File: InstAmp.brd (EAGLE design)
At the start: 77.5 x 18 mm, 37 parts, among them IC1 AD8221ARZ, IC2 TLC2254ID

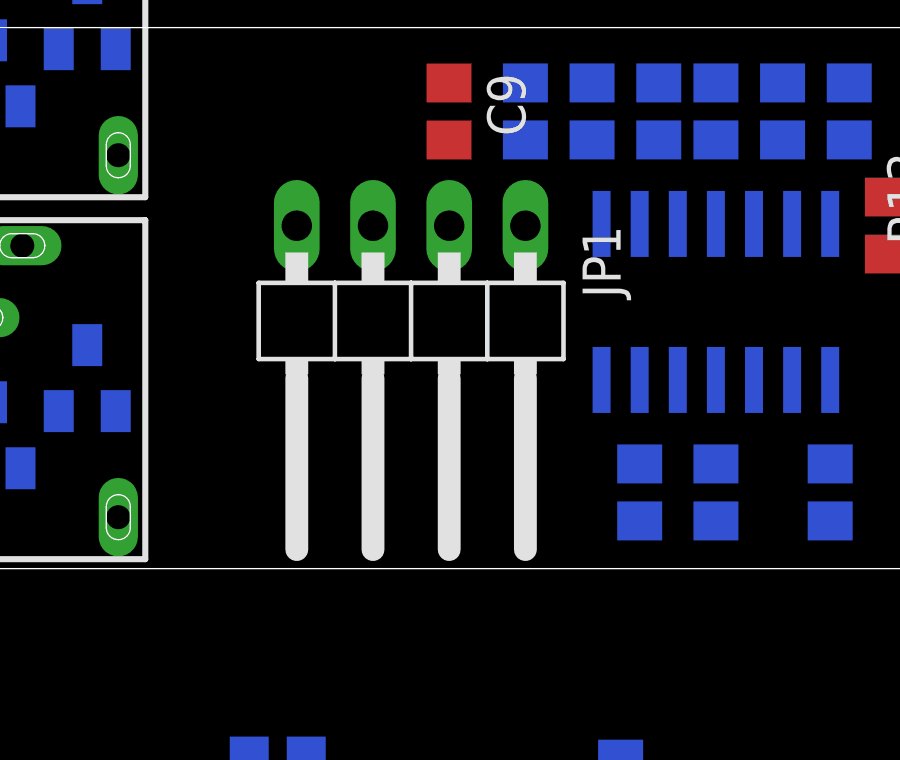
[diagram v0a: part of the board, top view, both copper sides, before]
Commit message: Amp routing
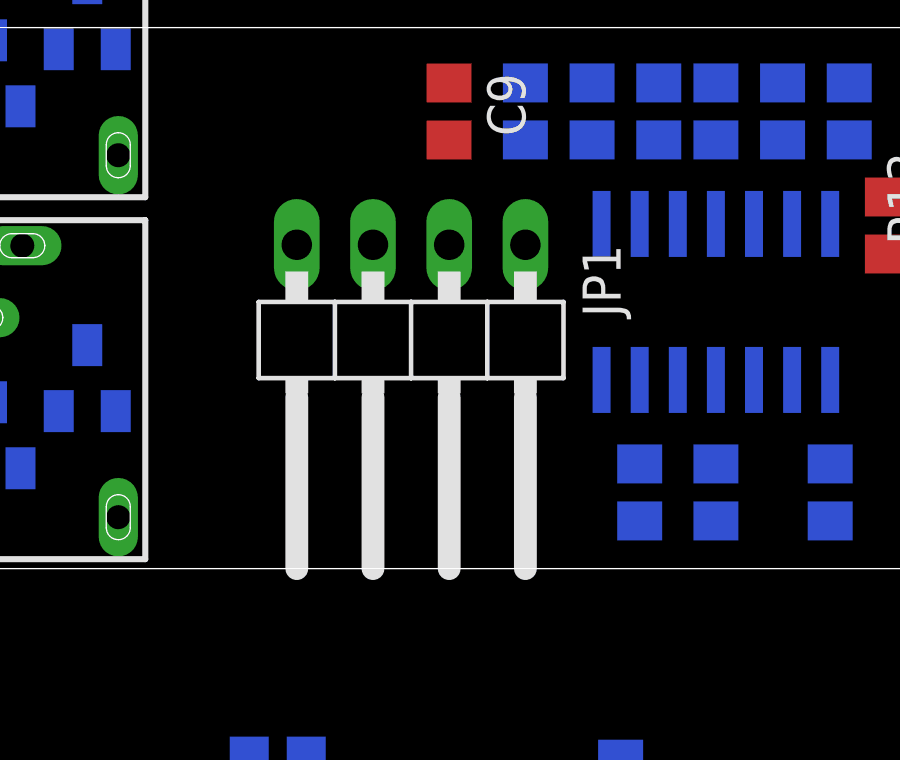
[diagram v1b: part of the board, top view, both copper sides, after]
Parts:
- moved JP1 0.63 mm to (22.9, 6.99)
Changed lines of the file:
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@@
 <element name="R16" library="rcl" package="R0805" value="910k" x="38.735" y="11.43" rot="R270"/>
 <element name="R17" library="rcl" package="R0805" value="100k" x="37.465" y="15.24" rot="MR270"/>
-<element name="JP1" library="pinhead" package="1X04/90" value="OUT" x="22.86" y="7.62" rot="R180"/>
+<element name="JP1" library="pinhead" package="1X04/90" value="OUT" x="22.86" y="6.985" rot="R180"/>
 <element name="IC2" library="linear" package="SO14" value="TLC2254ID" x="33.02" y="8.89" rot="MR180"/>
 </elements>
@@
 <wire x1="31.115" y1="16.19" x2="33.02" y2="16.19" width="0" layer="19" extent="16-16"/>
 <wire x1="28.8925" y1="16.19" x2="31.115" y2="16.19" width="0" layer="19" extent="16-16"/>
-<wire x1="24.13" y1="11.43" x2="28.8925" y2="16.19" width="0" layer="19" extent="16-16"/>
-<wire x1="30.48" y1="1.59" x2="24.13" y2="11.43" width="0" layer="19" extent="16-16"/>
+<wire x1="24.13" y1="10.795" x2="28.8925" y2="16.19" width="0" layer="19" extent="16-16"/>
+<wire x1="30.48" y1="1.59" x2="24.13" y2="10.795" width="0" layer="19" extent="16-16"/>
 <wire x1="33.02" y1="1.59" x2="30.48" y2="1.59" width="0" layer="19" extent="16-16"/>
 <wire x1="36.83" y1="1.59" x2="33.02" y2="1.59" width="0" layer="19" extent="16-16"/>
@@
 <wire x1="29.845" y1="-10.48" x2="29.845" y2="-8.2525" width="0" layer="19" extent="16-16"/>
 <wire x1="27.365" y1="-8.89" x2="29.845" y2="-8.2525" width="0" layer="19" extent="16-16"/>
-<wire x1="4.13" y1="5.715" x2="24.13" y2="11.43" width="0" layer="19" extent="16-16"/>
+<wire x1="4.13" y1="5.715" x2="24.13" y2="10.795" width="0" layer="19" extent="16-16"/>
 <wire x1="2.1" y1="5.715" x2="4.13" y2="5.715" width="0" layer="19" extent="16-16"/>
 <wire x1="4.13" y1="17.78" x2="4.13" y2="5.715" width="0" layer="19" extent="16-16"/>
@@
 <wire x1="29.845" y1="-6.3525" x2="33.02" y2="3.49" width="0" layer="19" extent="16-16"/>
 <wire x1="27.365" y1="-7.62" x2="29.845" y2="-6.3525" width="0" layer="19" extent="16-16"/>
-<wire x1="19.05" y1="11.43" x2="33.02" y2="6.29" width="0" layer="19" extent="16-16"/>
-<wire x1="13.015" y1="17.315" x2="19.05" y2="11.43" width="0" layer="19" extent="16-16"/>
+<wire x1="19.05" y1="10.795" x2="33.02" y2="6.29" width="0" layer="19" extent="16-16"/>
+<wire x1="13.015" y1="17.315" x2="19.05" y2="10.795" width="0" layer="19" extent="16-16"/>
 <wire x1="9.84" y1="15.41" x2="13.015" y2="17.315" width="0" layer="19" extent="16-16"/>
-<wire x1="13.015" y1="5.25" x2="19.05" y2="11.43" width="0" layer="19" extent="16-16"/>
+<wire x1="13.015" y1="5.25" x2="19.05" y2="10.795" width="0" layer="19" extent="16-16"/>
 <wire x1="9.84" y1="3.345" x2="13.015" y2="5.25" width="0" layer="19" extent="16-16"/>
 </signal>
@@
 <contactref element="IC2" pad="4"/>
 <wire x1="33.02" y1="11.49" x2="33.02" y2="14.29" width="0" layer="19" extent="16-16"/>
-<wire x1="21.59" y1="11.43" x2="33.02" y2="11.49" width="0" layer="19" extent="16-16"/>
-<wire x1="11.115" y1="17.315" x2="21.59" y2="11.43" width="0" layer="19" extent="16-16"/>
+<wire x1="21.59" y1="10.795" x2="33.02" y2="11.49" width="0" layer="19" extent="16-16"/>
+<wire x1="11.115" y1="17.315" x2="21.59" y2="10.795" width="0" layer="19" extent="16-16"/>
 <wire x1="7.94" y1="15.41" x2="11.115" y2="17.315" width="0" layer="19" extent="16-16"/>
 <wire x1="11.115" y1="5.25" x2="7.94" y2="15.41" width="0" layer="19" extent="16-16"/>
@@
 <contactref element="C9" pad="2"/>
 <wire x1="24.13" y1="14.29" x2="26.67" y2="14.29" width="0" layer="19" extent="1-16"/>
-<wire x1="26.67" y1="11.43" x2="26.67" y2="14.29" width="0" layer="19" extent="16-16"/>
-<wire x1="29.21" y1="11.49" x2="26.67" y2="11.43" width="0" layer="19" extent="16-16"/>
+<wire x1="26.67" y1="10.795" x2="26.67" y2="14.29" width="0" layer="19" extent="16-16"/>
+<wire x1="29.21" y1="11.49" x2="26.67" y2="10.795" width="0" layer="19" extent="16-16"/>
 </signal>
 <signal name="N$20">

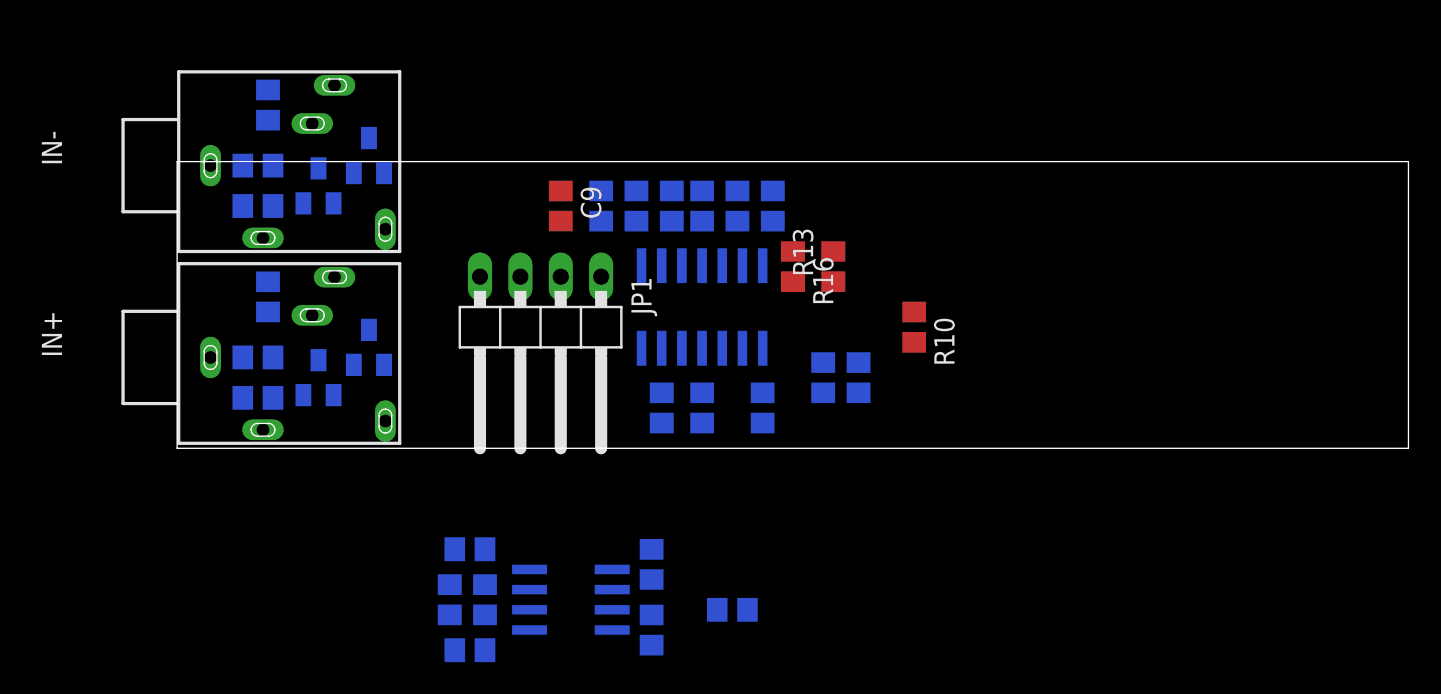
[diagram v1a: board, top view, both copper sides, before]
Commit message: Better comps
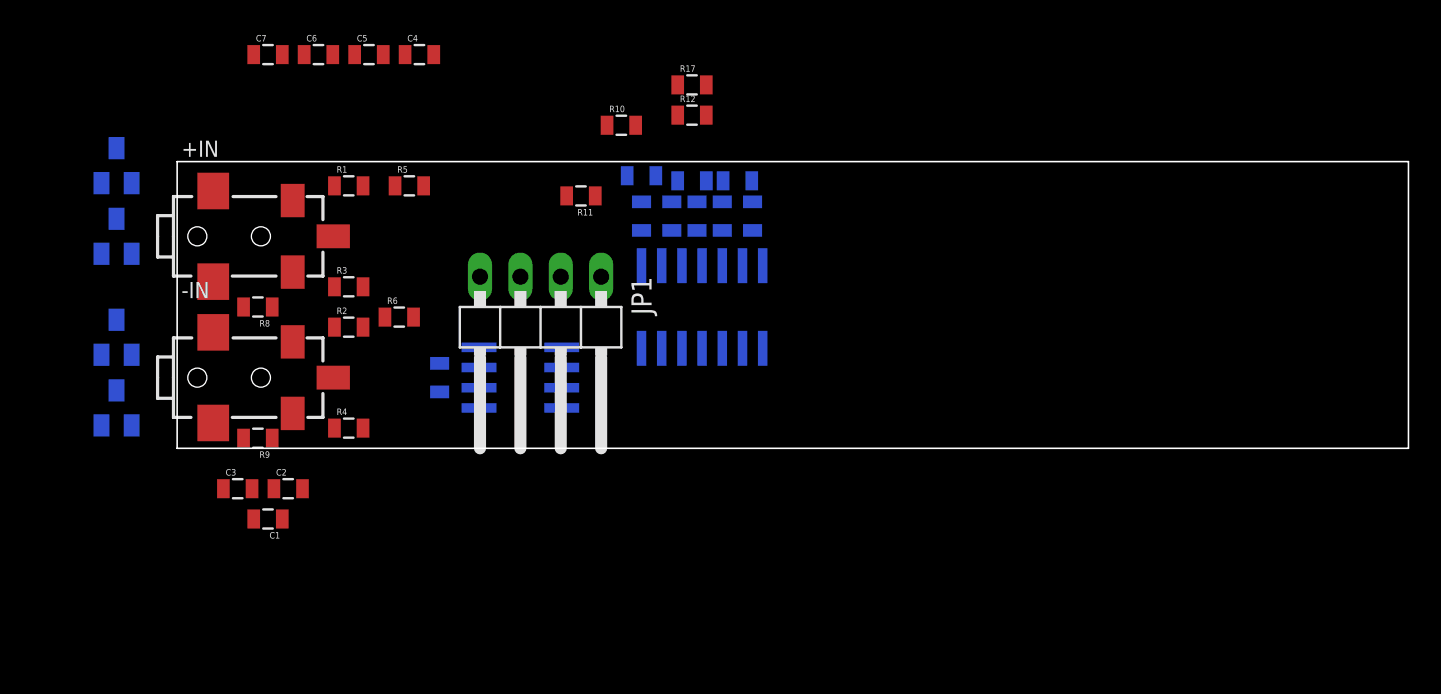
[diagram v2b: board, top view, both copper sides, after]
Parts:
- removed IN+, IN-: 1503_09, con-lumberg:1503_09
- added +IN, -IN: (no value), SparkFun-Connectors:STEREOJACK2.5MM_SMD
- C1, C10, C11, C2, C3, C8, C9: device rcl:C0805 -> SparkFun-Passives:0805
- C4, C5, C6, C7: value 0.1uF -> 100nF; device rcl:C0805 -> SparkFun-Passives:0805
- R1, R10, R11, R12, R13, R14, R15, R16, R17, R2, R3, R4, R5, R6, R7, R8, R9: device rcl:R0805 -> SparkFun-Passives:0805
- moved C5 40.3 mm to (12.1, 24.8), flipped to the top, turned to 0 degrees
- moved C4 35.2 mm to (15.2, 24.8), flipped to the top, turned to 0 degrees
- moved C7 35.2 mm to (5.71, 24.8), flipped to the top, turned to 0 degrees
- moved R8 32.4 mm to (5.08, 8.89), flipped to the top, turned to 180 degrees
- moved R5 29.5 mm to (14.6, 16.5), flipped to the top, turned to 0 degrees
- moved C6 25.9 mm to (8.89, 24.8), flipped to the top, turned to 0 degrees
- moved R9 25.5 mm to (5.08, 0.64), flipped to the top, turned to 180 degrees
- moved C11 24.8 mm to (34.3, 14.6), turned to 270 degrees
- moved R10 22.4 mm to (27.9, 20.3), turned to 0 degrees
- moved R4 20.9 mm to (10.8, 1.27), flipped to the top, turned to 0 degrees
- moved C3 20.4 mm to (3.81, -2.54), flipped to the top, turned to 0 degrees
- moved D4 16.7 mm to (-3.81, 13.3)
- moved D2 16.3 mm to (-3.81, 2.54)
- moved R6 15.3 mm to (14.0, 8.26), flipped to the top, turned to 0 degrees
- moved C10 14.9 mm to (32.4, 16.8), turned to 180 degrees
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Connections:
- net GND: now also +IN.5, -IN.5; no longer IN+.1, IN-.1
- net N$1: now also -IN.1; no longer IN-.2
- net N$11: now also C10.1; no longer C11.2
- net N$2: now also -IN.4; no longer IN-.3
- net N$22: now also C11.2; no longer C10.1
- net N$3: now also +IN.1, R1.1; no longer IN+.3, R3.1
- net N$4: now also +IN.4, R3.1; no longer IN+.2, R1.1

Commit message: .
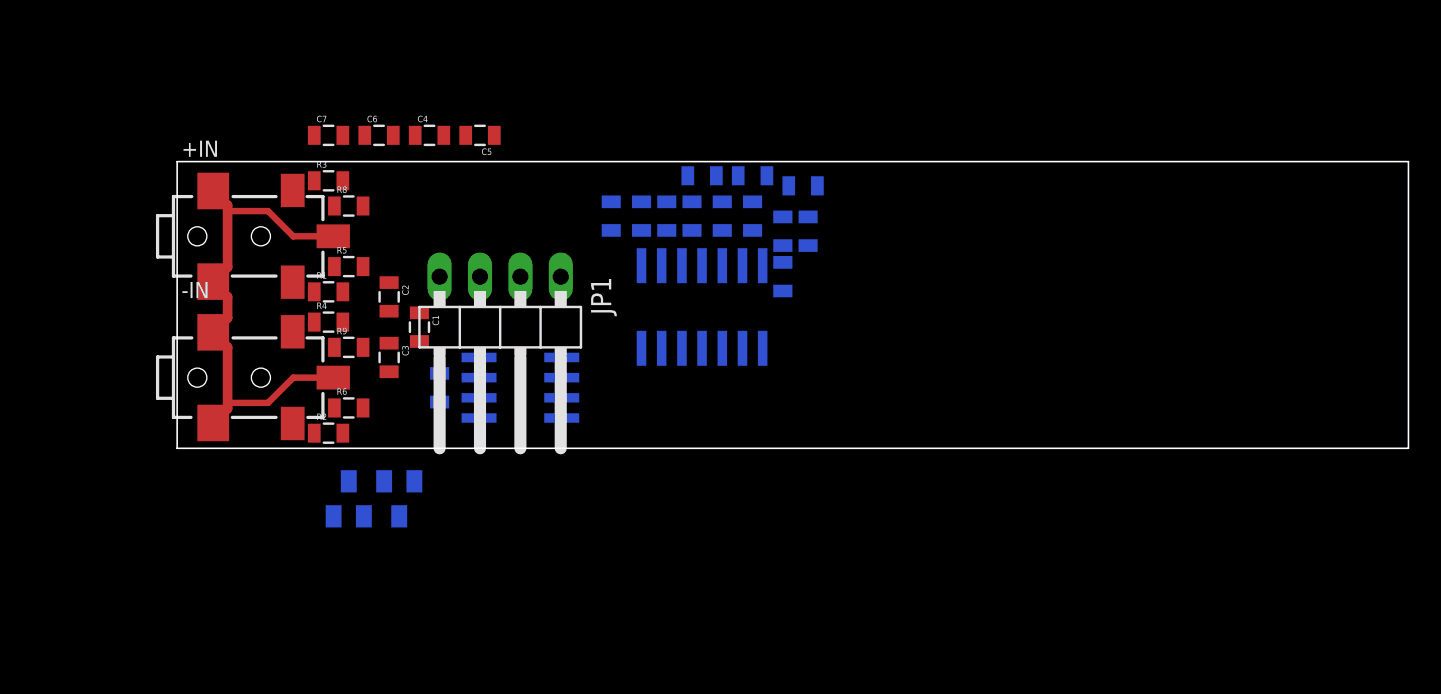
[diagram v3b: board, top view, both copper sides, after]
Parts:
- removed D3, D4: BAV199, diode:SOT23
- +IN, -IN: value (none) -> AUDIOJACK2.5-SMD; device SparkFun-Connectors:STEREOJACK2.5MM_SMD -> femtoexg:AUDIOJACK2.5-SMD
- D1, D2: device diode:SOT23 -> SparkFun-DiscreteSemi:SOT23
- moved D1 20.5 mm to (14.0, -3.17), turned to 180 degrees
- moved D2 15.7 mm to (10.8, -3.17)
- moved C1 15.4 mm to (15.2, 7.62), turned to 270 degrees
- moved C2 13.6 mm to (13.3, 9.53), turned to 270 degrees
- moved C3 12.6 mm to (13.3, 5.71), turned to 270 degrees
- moved R17 9.09 mm to (36.2, 14.6), flipped to the bottom, turned to 270 degrees
- moved C5 8.64 mm to (19.1, 19.7), turned to 180 degrees
- moved R8 8.54 mm to (10.8, 15.2), turned to 0 degrees
- moved R9 8.08 mm to (10.8, 6.35), turned to 0 degrees
- moved C10 7.96 mm to (39.7, 13.7), turned to 90 degrees
- moved R13 6.98 mm to (36.2, 17.1)
- moved R1 6.79 mm to (9.53, 9.84)
- moved R2 6.79 mm to (9.53, 0.95)
- moved R3 6.79 mm to (9.53, 16.8)
- moved R4 6.79 mm to (9.53, 7.94)
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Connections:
- net +5V: no longer D3.2, D4.2
- net -5V: no longer D3.1, D4.1
- net GND: now also +IN.GND1, +IN.GND2, +IN.SW, -IN.GND1, -IN.GND2, -IN.SW; no longer +IN.5, -IN.5
- net N$1: now also +IN.L, R1.1; no longer -IN.1, R2.1
- net N$17: no longer D2.3
- net N$2: now also -IN.R; no longer -IN.4
- net N$3: now also +IN.R, R3.1; no longer +IN.1, R1.1
- net N$4: now also -IN.L, R2.1; no longer +IN.4, R3.1
- net N$5: now also D2.3; no longer D3.3
- net N$7: no longer D4.3
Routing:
- net GND: track 0.00 -> 31.5 mm

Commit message: .
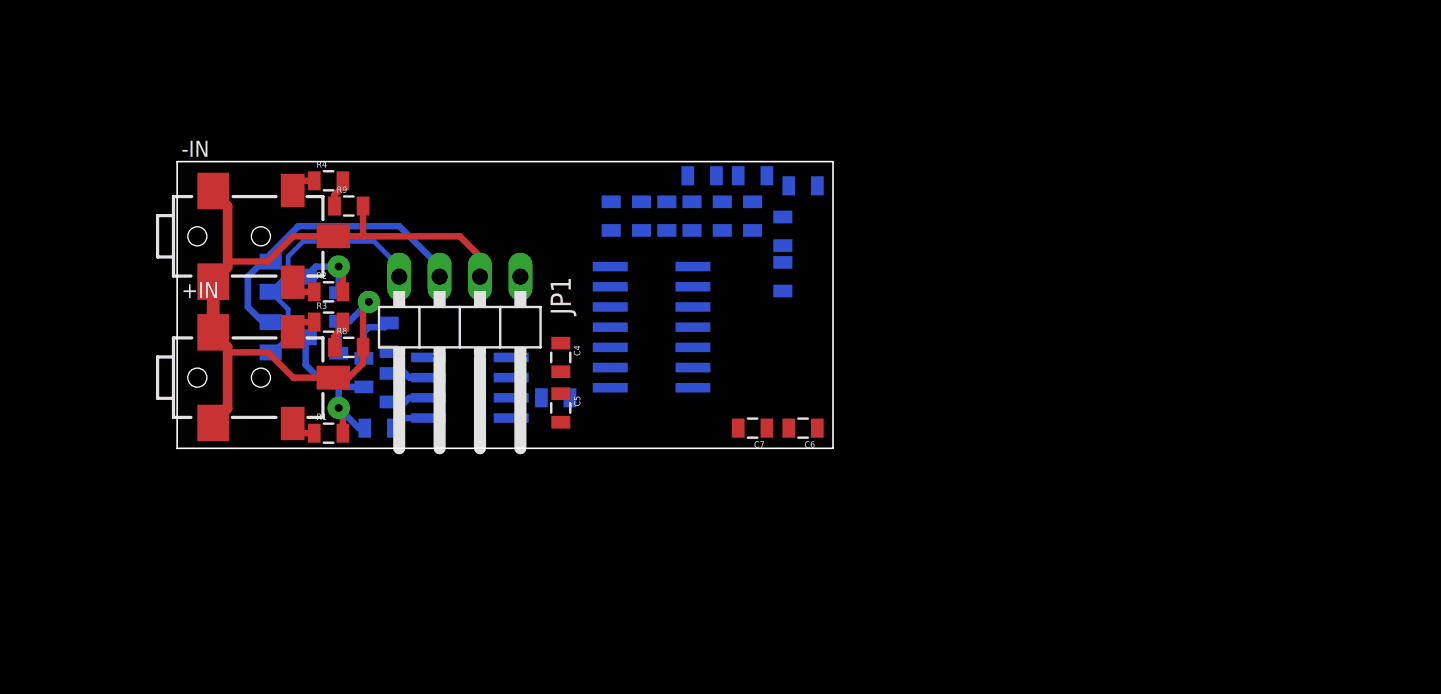
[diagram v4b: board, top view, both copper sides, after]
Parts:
- moved C7 32.4 mm to (36.2, 1.27), turned to 180 degrees
- moved C6 32.4 mm to (39.4, 1.27), turned to 180 degrees
- moved C10 19.0 mm to (23.8, 3.17), turned to 180 degrees
- moved C5 17.9 mm to (24.1, 2.54), turned to 270 degrees
- moved C4 16.2 mm to (24.1, 5.71), turned to 270 degrees
- moved D2 14.5 mm to (6.99, 10.8), turned to 90 degrees
- moved D1 12.3 mm to (6.99, 6.99), turned to 90 degrees
- moved R5 10.3 mm to (12.7, 1.27), flipped to the bottom, turned to 180 degrees
- moved +IN 8.89 mm to (1.27, 4.45)
- moved -IN 8.89 mm to (1.27, 13.3)
- moved R3 8.89 mm to (9.53, 7.94)
- moved R4 8.89 mm to (9.53, 16.8)
- moved R8 8.89 mm to (10.8, 6.35)
- moved R9 8.89 mm to (10.8, 15.2)
- moved R1 8.89 mm to (9.53, 0.95)
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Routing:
- net GND: track 31.5 -> 55.3 mm, vias 0 -> 1
- net +5V: track 0.00 -> 19.1 mm
- net -5V: track 0.00 -> 16.2 mm
- net N$6: track 0.00 -> 11.5 mm, vias 0 -> 1
- net N$5: track 0.00 -> 9.14 mm, vias 0 -> 1
- net N$8: track 0.00 -> 2.63 mm
- net N$16: track 0.00 -> 2.63 mm
- net N$12: track 0.00 -> 2.48 mm
- net N$7: track 0.00 -> 1.81 mm
- net N$17: track 0.00 -> 1.81 mm
- net N$2: track 0.00 -> 1.61 mm
- net N$4: track 0.00 -> 1.61 mm
- net N$3: track 0.00 -> 1.61 mm
- net N$1: track 0.00 -> 1.61 mm
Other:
- board size 77.5 x 18 mm -> 41.3 x 18 mm
